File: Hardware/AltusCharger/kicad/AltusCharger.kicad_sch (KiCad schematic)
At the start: 70 parts, among them J1 Conn_01x02_Socket, J2 Conn_01x02_Socket, J3 USB_C_Receptacle_USB2.0_16P, J4 Conn_01x02_Socket, J5 Conn_01x02_Socket, J6 Conn_01x02_Socket, J7 Conn_01x02_Socket, Q1 AO3401A, Q2 AO3400A, Q3 AO3400A, SW1 SSSS811101, U1 MCP73831-2-OT, U2 MCP73831-2-OT, U3 MCP73831-2-OT, U4 MCP73831-2-OT, U5 MCP73831-2-OT, U6 MCP73831-2-OT

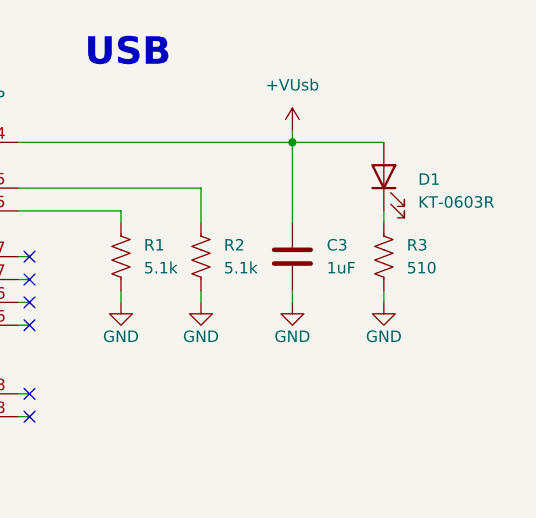
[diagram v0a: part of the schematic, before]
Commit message: Altus Charger V1.0
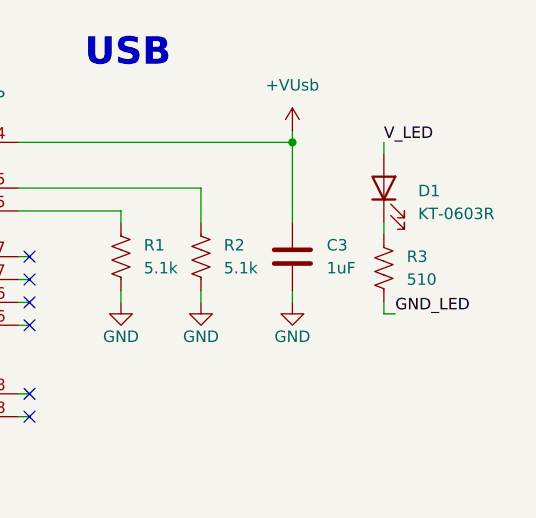
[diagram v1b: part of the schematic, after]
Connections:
- net +VUsb: no longer D1.2 (A)
- net GND: no longer R3.2
- net GND_LED: now also R3.2
- net V_LED: now also D1.2 (A)
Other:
- moved on the sheet: D1, R3
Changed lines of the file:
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@@
 	(wire
 		(pts
-			(xy 259.08 27.94) (xy 269.24 27.94)
-		)
-		(stroke
-			(width 0)
-			(type default)
-		)
-	)
-	(wire
-		(pts
 			(xy 101.6 135.89) (xy 101.6 137.16)
 		)
@@
 	(wire
 		(pts
-			(xy 269.24 35.56) (xy 269.24 36.83)
+			(xy 269.24 27.94) (xy 269.24 29.21)
 		)
 		(stroke
@@
 	(wire
 		(pts
-			(xy 269.24 44.45) (xy 269.24 45.72)
-		)
-		(stroke
-			(width 0)
-			(type default)
-		)
-	)
-	(wire
-		(pts
 			(xy 101.6 52.07) (xy 101.6 50.8)
 		)
@@
 	(wire
 		(pts
+			(xy 269.24 46.99) (xy 269.24 45.72)
+		)
+		(stroke
+			(width 0)
+			(type default)
+		)
+	)
+	(wire
+		(pts
 			(xy 101.6 34.29) (xy 101.6 35.56)
 		)
@@
 	(wire
 		(pts
+			(xy 270.51 46.99) (xy 269.24 46.99)
+		)
+		(stroke
+			(width 0)
+			(type default)
+		)
+	)
+	(wire
+		(pts
 			(xy 38.1 127) (xy 38.1 133.35)
 		)
@@
 	(wire
 		(pts
+			(xy 269.24 36.83) (xy 269.24 38.1)
+		)
+		(stroke
+			(width 0)
+			(type default)
+		)
+	)
+	(wire
+		(pts
 			(xy 69.85 43.18) (xy 69.85 44.45)
 		)
@@
 	)
 	(label "GND_LED"
+		(at 270.51 46.99 0)
+		(effects
+			(font
+				(size 1.27 1.27)
+			)
+			(justify left bottom)
+		)
+	)
+	(label "GND_LED"
 		(at 128.27 165.1 0)
 		(effects
@@
 	)
 	(label "V_LED"
+		(at 269.24 27.94 0)
+		(effects
+			(font
+				(size 1.27 1.27)
+			)
+			(justify left bottom)
+		)
+	)
+	(label "V_LED"
 		(at 146.05 93.98 0)
 		(effects
@@
 	(symbol
 		(lib_id "Device:R_US")
-		(at 269.24 40.64 0)
+		(at 269.24 41.91 0)
 		(unit 1)
 		(exclude_from_sim no)
@@
 		(fields_autoplaced yes)
 		(property "Reference" "R3"
-			(at 271.78 39.3699 0)
+			(at 271.78 40.6399 0)
 			(effects
 				(font
@@
 		)
 		(property "Value" "510"
-			(at 271.78 41.9099 0)
+			(at 271.78 43.1799 0)
 			(effects
 				(font
@@
 		)
 		(property "Footprint" "Resistor_SMD:R_0402_1005Metric"
-			(at 270.256 40.894 90)
+			(at 270.256 42.164 90)
 			(effects
 				(font
@@
 		)
 		(property "Datasheet" "https://jlcpcb.com/api/file/downloadByFileSystemAccessId/8579706044791963648"
-			(at 269.24 40.64 0)
+			(at 269.24 41.91 0)
 			(effects
 				(font
@@
 		)
 		(property "Description" "Resistor, US symbol"
-			(at 269.24 40.64 0)
+			(at 269.24 41.91 0)
 			(effects
 				(font
@@
 		)
 		(property "JLCPCB Part #" "C25123"
-			(at 269.24 40.64 0)
+			(at 269.24 41.91 0)
 			(effects
 				(font
@@
 		(lib_name "LED_1")
 		(lib_id "Device:LED")
-		(at 269.24 31.75 90)
+		(at 269.24 33.02 90)
 		(unit 1)
 		(exclude_from_sim no)
@@
 		(fields_autoplaced yes)
 		(property "Reference" "D1"
-			(at 273.05 32.0674 90)
+			(at 273.05 33.3374 90)
 			(effects
 				(font
@@
 		)
 		(property "Value" "KT-0603R"
-			(at 273.05 34.6074 90)
+			(at 273.05 35.8774 90)
 			(effects
 				(font
@@
 		)
 		(property "Footprint" "LED_SMD:LED_0603_1608Metric"
-			(at 269.24 31.75 0)
+			(at 269.24 33.02 0)
 			(effects
 				(font
@@
 		)
 		(property "Datasheet" "~"
-			(at 269.24 31.75 0)
+			(at 269.24 33.02 0)
 			(effects
 				(font
@@
 		)
 		(property "Description" "Light emitting diode"
-			(at 269.24 31.75 0)
+			(at 269.24 33.02 0)
 			(effects
 				(font
@@
 		)
 		(property "JLCPCB Part #" "C2286"
-			(at 269.24 31.75 0)
+			(at 269.24 33.02 0)
 			(effects
 				(font
@@
 		)
 		(property "Sim.Pins" "1=K 2=A"
-			(at 269.24 31.75 0)
+			(at 269.24 33.02 0)
 			(effects
 				(font
@@
 					(unit 1)
 				)
-			)
-		)
-	)
-	(symbol
-		(lib_id "power:GND")
-		(at 269.24 45.72 0)
-		(unit 1)
-		(exclude_from_sim no)
-		(in_bom yes)
-		(on_board yes)
-		(dnp no)
-		(property "Reference" "#PWR011"
-			(at 269.24 52.07 0)
-			(effects
-				(font
-					(size 1.27 1.27)
-				)
-				(hide yes)
-			)
-		)
-		(property "Value" "GND"
-			(at 269.24 49.53 0)
-			(effects
-				(font
-					(size 1.27 1.27)
-				)
-			)
-		)
-		(property "Footprint" ""
-			(at 269.24 45.72 0)
-			(effects
-				(font
-					(size 1.27 1.27)
-				)
-				(hide yes)
-			)
-		)
-		(property "Datasheet" ""
-			(at 269.24 45.72 0)
-			(effects
-				(font
-					(size 1.27 1.27)
-				)
-				(hide yes)
-			)
-		)
-		(property "Description" "Power symbol creates a global label with name \"GND\" , ground"
-			(at 269.24 45.72 0)
-			(effects
-				(font
-					(size 1.27 1.27)
-				)
-				(hide yes)
-			)
-		)
-		(pin "1"
-		)
-		(instances
-			(project "AltusCharger"
-				(path "/fb372b2b-e129-460a-8a5a-84eeae8ddbd5"
-					(reference "#PWR011")
-					(unit 1)
-				)
